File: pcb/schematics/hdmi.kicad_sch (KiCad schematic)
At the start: 18 parts, among them J8 HDMI_A, U6 TFP410PAP, U7 ESD224DQA, U8 ESD224DQA

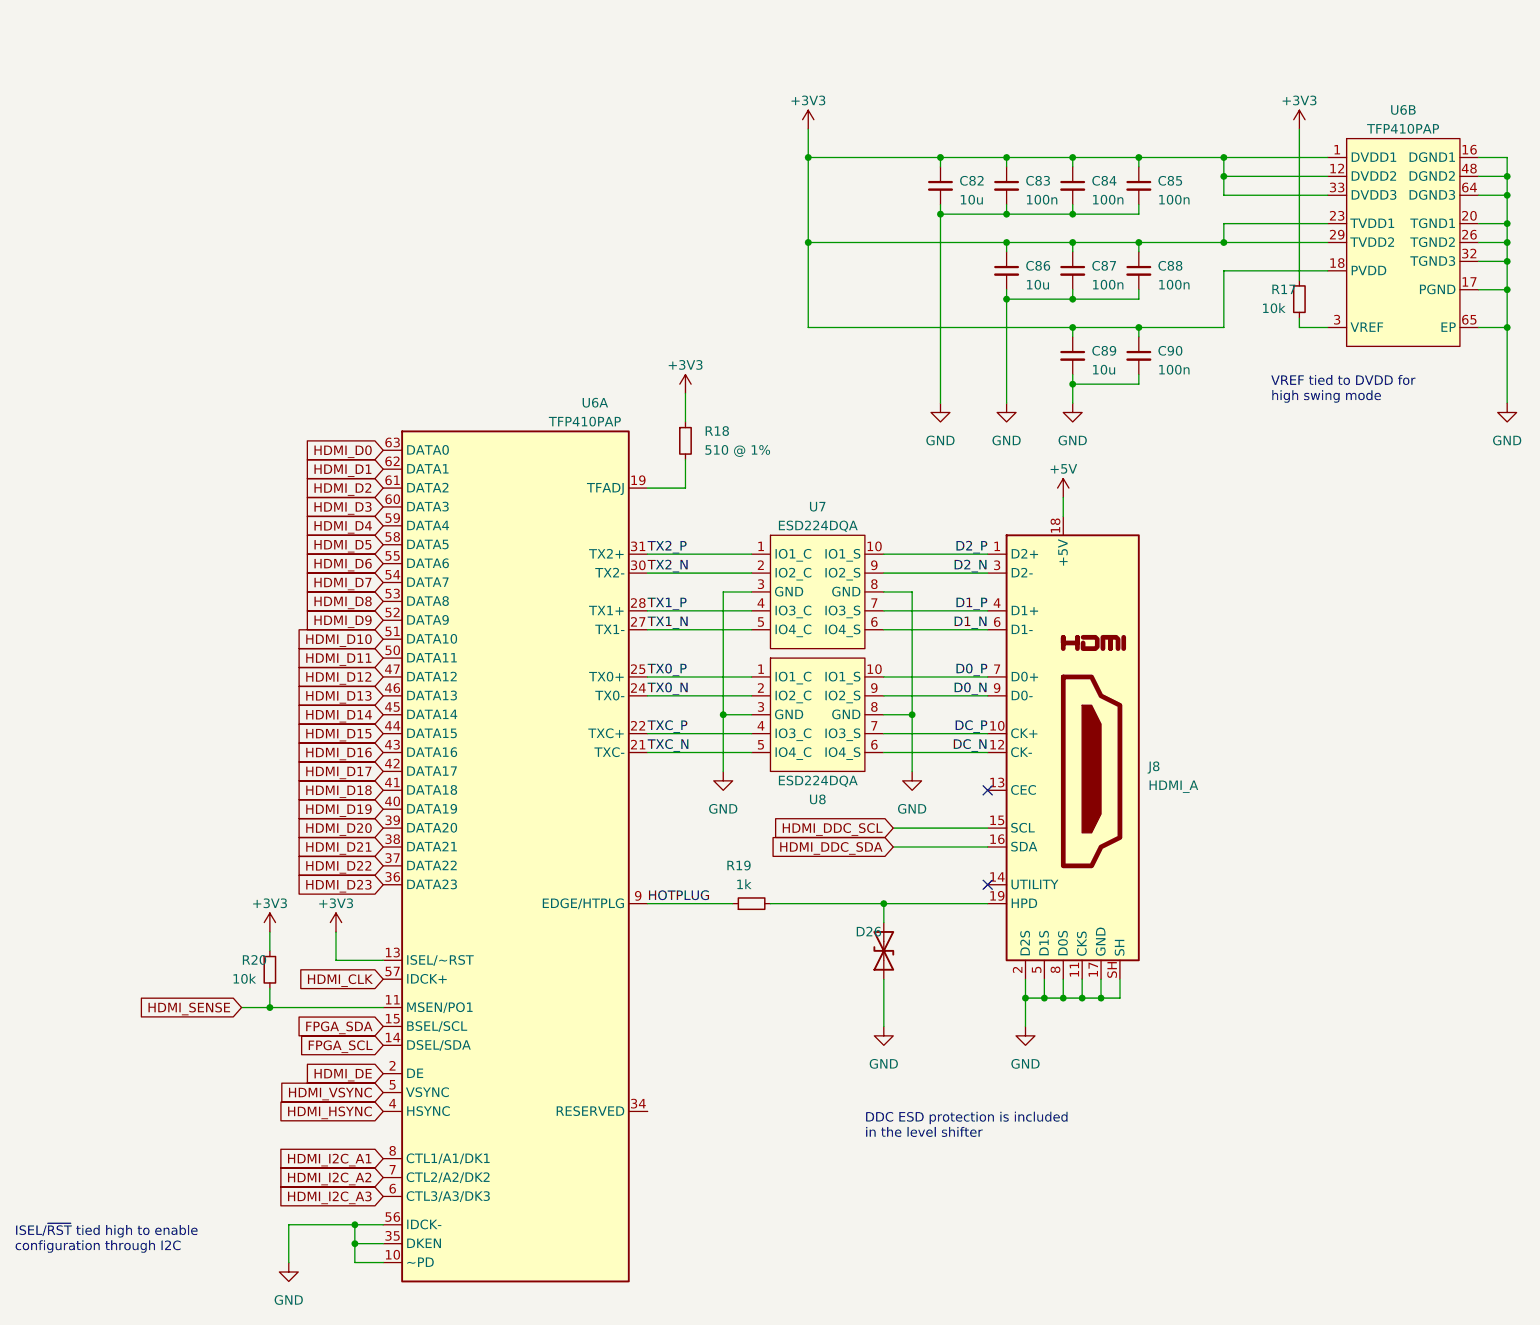
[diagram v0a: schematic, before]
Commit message: add shield
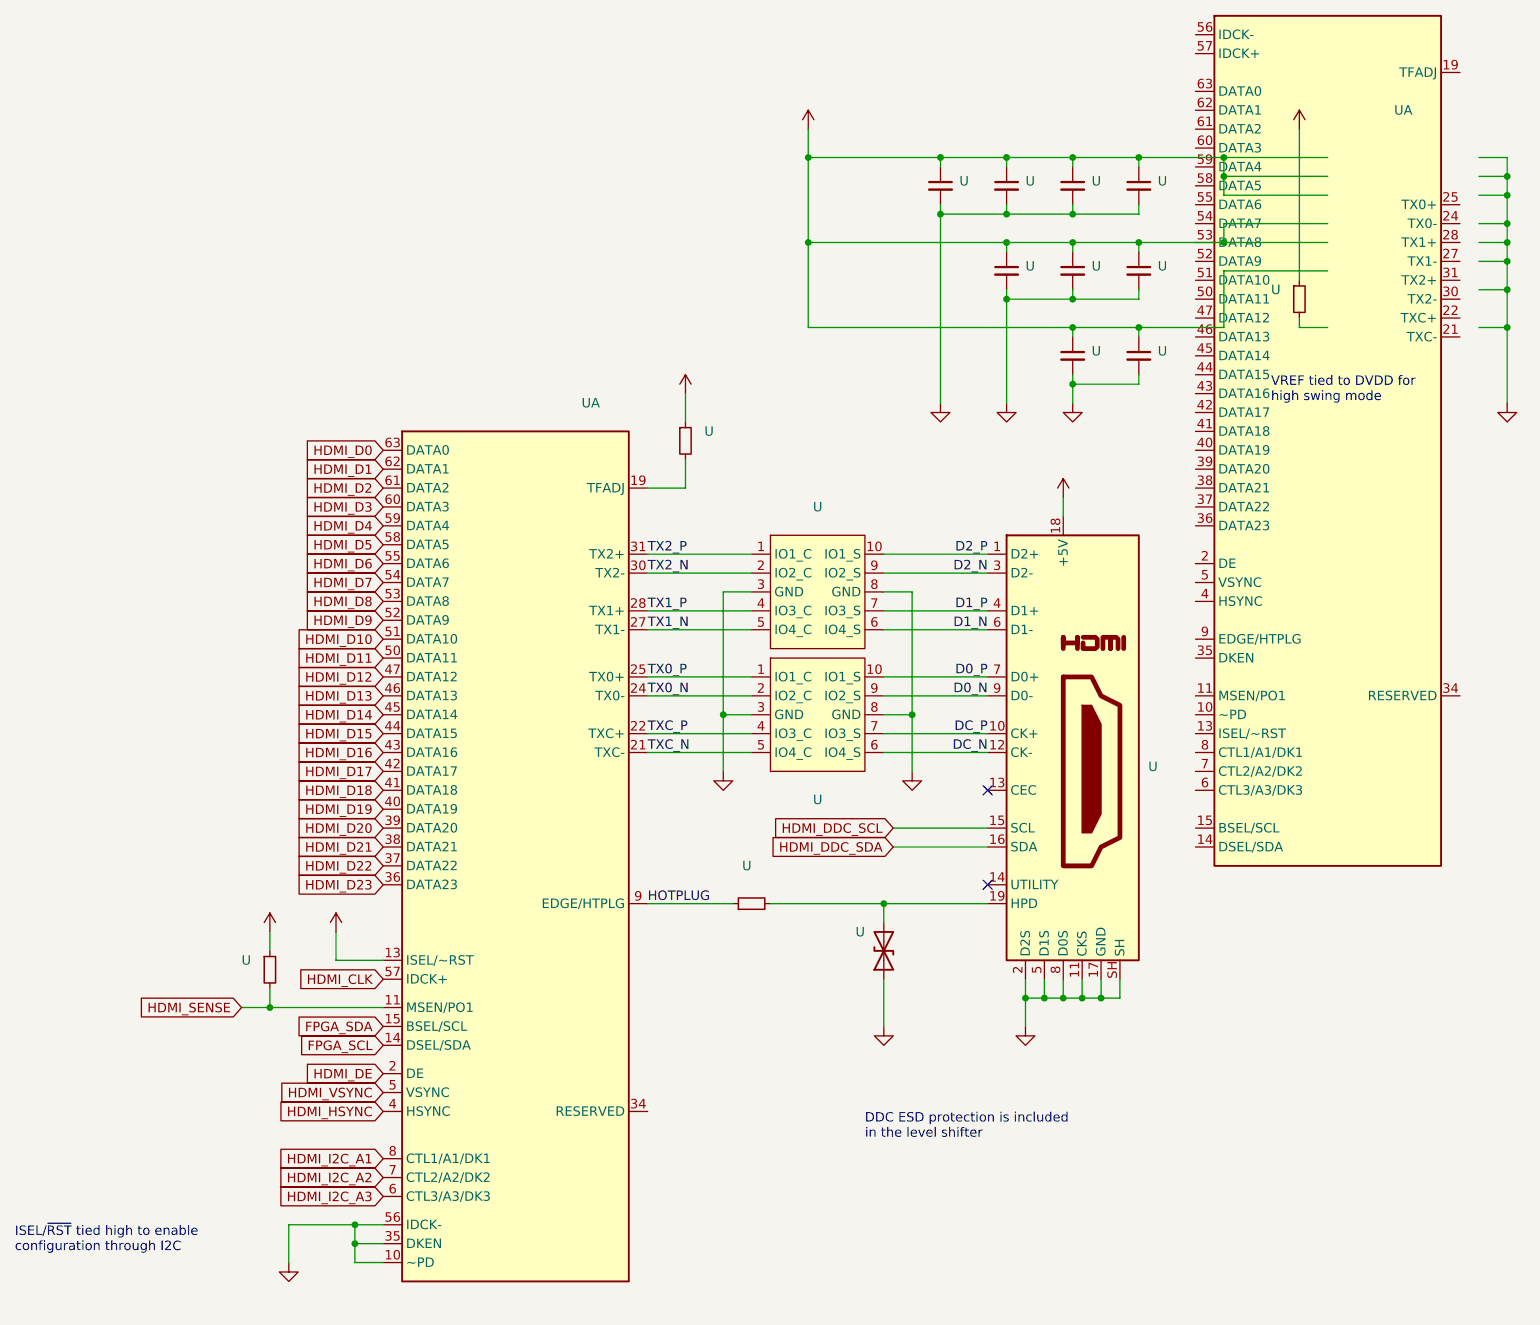
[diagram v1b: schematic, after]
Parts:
- U: renamed from J8; value HDMI_A -> (none); footprint RAHHD19TR:RAAHD19TR -> (none)
- U: renamed from C89; value 10u -> (none); footprint Capacitor_SMD:C_0805_2012Metric -> (none)
- U: renamed from C83; value 100n -> (none); footprint Capacitor_SMD:C_0603_1608Metric -> (none)
- U: renamed from R20; value 10k -> (none); footprint Resistor_SMD:R_0603_1608Metric -> (none)
- U: renamed from C82; value 10u -> (none); footprint Capacitor_SMD:C_0805_2012Metric -> (none)
- U: renamed from C86; value 10u -> (none); footprint Capacitor_SMD:C_0805_2012Metric -> (none)
- U: renamed from D26; value D_TVS -> (none); footprint Diode_SMD:D_0603_1608Metric -> (none)
- U: renamed from C87; value 100n -> (none); footprint Capacitor_SMD:C_0603_1608Metric -> (none)
- U: renamed from C84; value 100n -> (none); footprint Capacitor_SMD:C_0603_1608Metric -> (none)
- U: renamed from U6; value TFP410PAP -> (none); footprint Package_QFP:HTQFP-64-1EP_10x10mm_P0.5mm_EP8x8mm_Mask4.4x4.4mm_ThermalVias -> (none)
- U: renamed from U8; value ESD224DQA -> (none); footprint ESD224DQA:IC_TPD4EUSB30DQAR -> (none)
- U: renamed from C88; value 100n -> (none); footprint Capacitor_SMD:C_0603_1608Metric -> (none)
- U: renamed from C85; value 100n -> (none); footprint Capacitor_SMD:C_0603_1608Metric -> (none)
- U: renamed from R17; value 10k -> (none); footprint Resistor_SMD:R_0603_1608Metric -> (none)
- U: renamed from C90; value 100n -> (none); footprint Capacitor_SMD:C_0603_1608Metric -> (none)
- U: renamed from R18; value 510 @ 1% -> (none); footprint Resistor_SMD:R_0603_1608Metric -> (none)
- U: renamed from R19; value 1k -> (none); footprint Resistor_SMD:R_0603_1608Metric -> (none)
- U: renamed from U7; value ESD224DQA -> (none); footprint ESD224DQA:IC_TPD4EUSB30DQAR -> (none)
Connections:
- net +3V3: no longer U.1 (DVDD1), U.12 (DVDD2), U.18 (PVDD), U.23 (TVDD1), U.29 (TVDD2), U.33 (DVDD3)
- net GND: no longer U.16 (DGND1), U.17 (PGND), U.20 (TGND1), U.26 (TGND2), U.32 (TGND3), U.48 (DGND2), U.64 (DGND3), U.65 (EP)
- net at U.2: no longer U.3 (VREF)
